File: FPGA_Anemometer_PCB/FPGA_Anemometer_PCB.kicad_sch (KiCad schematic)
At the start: 7 parts, among them J3 YO0221500000G, J4 YO0221500000G

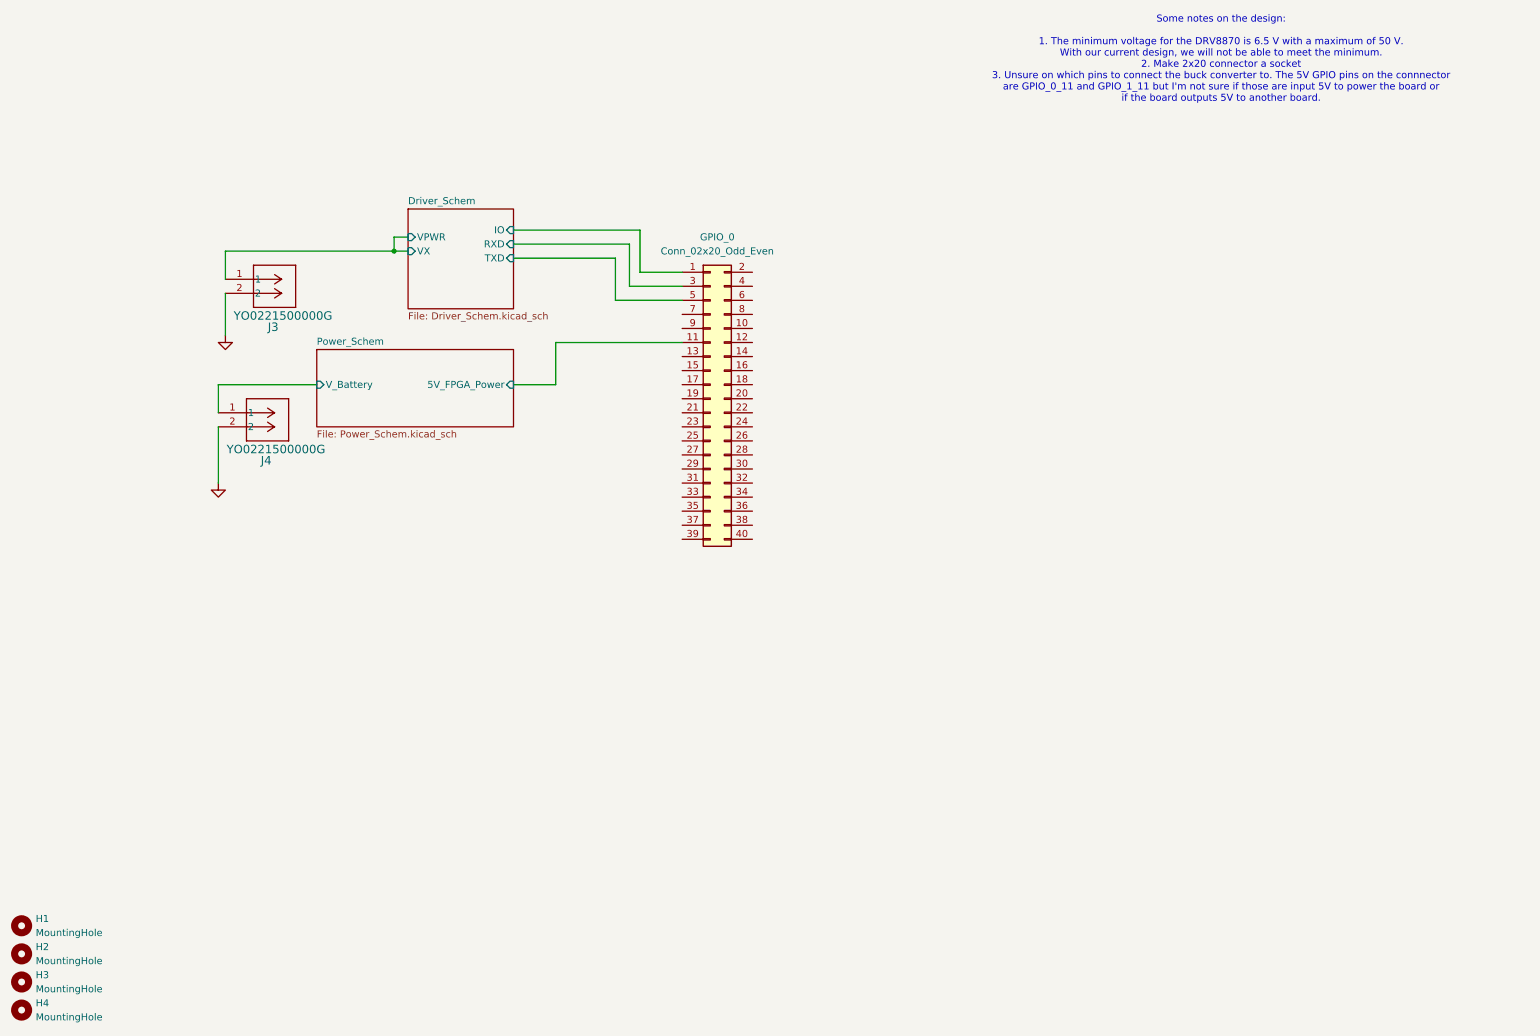
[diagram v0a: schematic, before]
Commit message: updated pcb
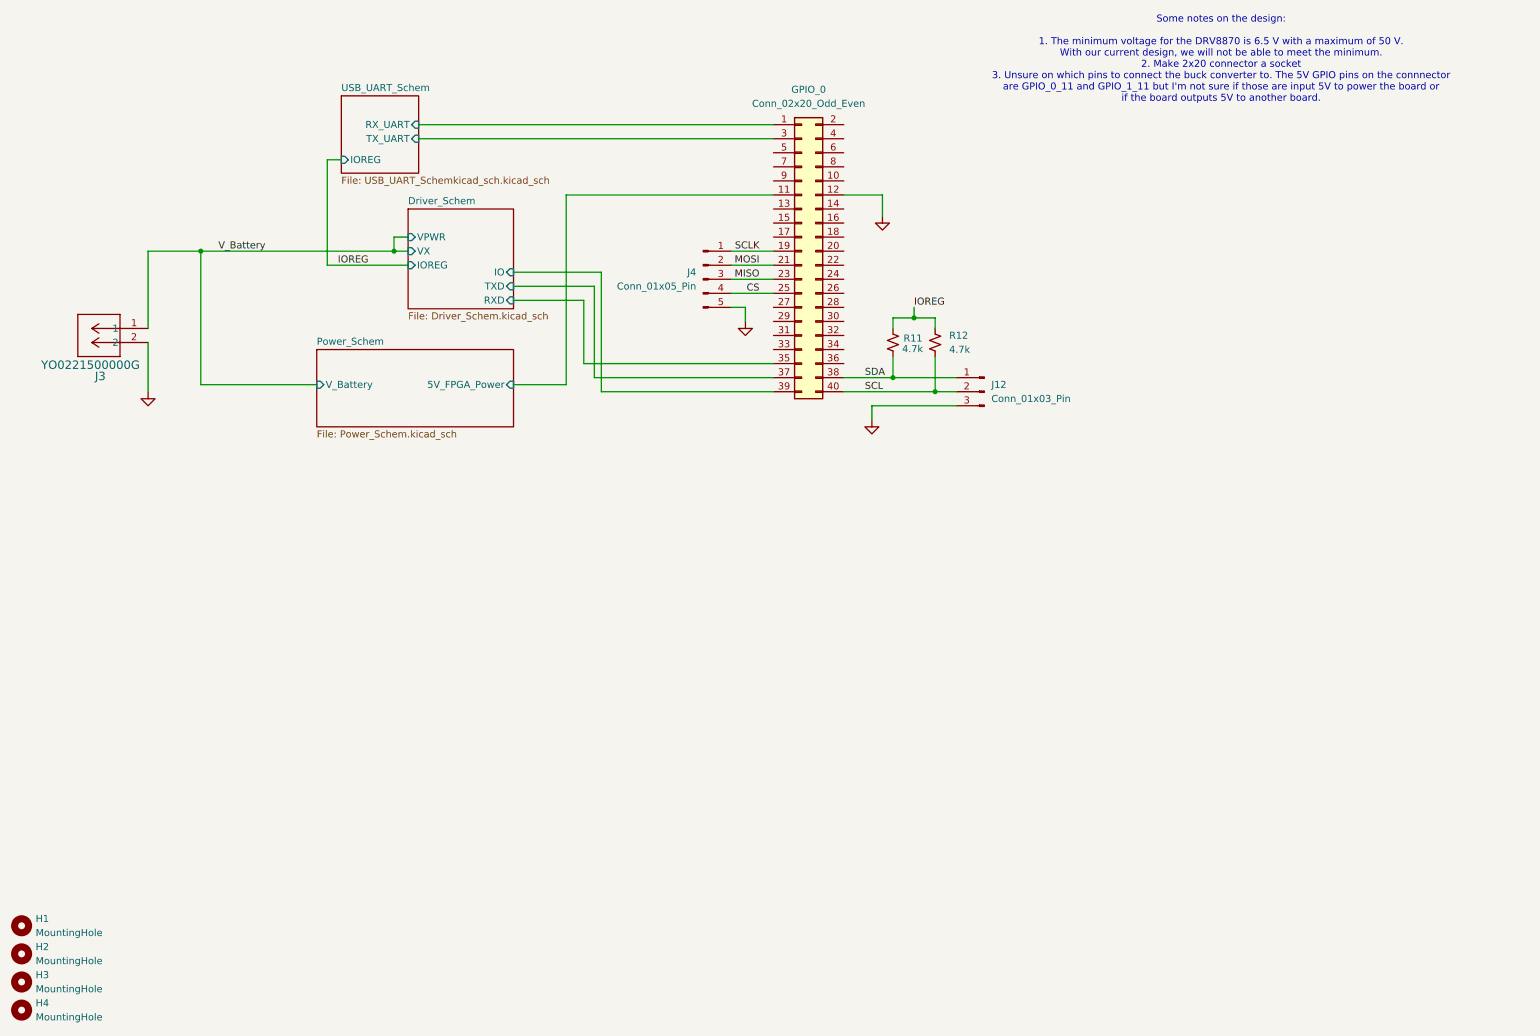
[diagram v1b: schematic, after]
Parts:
- removed J4: YO0221500000G, footprints:CONN_YO0221500000G_AMP, symbol 2026-01-23_14-54-26:YO0221500000G
- added J12: Conn_01x03_Pin, Connector_PinHeader_2.54mm:PinHeader_1x03_P2.54mm_Vertical, symbol Connector:Conn_01x03_Pin
- added J4: Conn_01x05_Pin, Connector_PinHeader_2.54mm:PinHeader_1x05_P2.54mm_Vertical, symbol Connector:Conn_01x05_Pin
- added R11, R12: 4.7k, Resistor_SMD:R_0805_2012Metric, symbol Device:R_Small_US
- J3: footprint footprints:CONN_YO0221500000G_AMP -> YO0221500000G:CONN_YO0221500000G_AMP
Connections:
- net Driver_Schem/IO: now also GPIO_0.39 (Pin_39); no longer GPIO_0.1 (Pin_1)
- net Driver_Schem/RXD: now also GPIO_0.35 (Pin_35); no longer GPIO_0.3 (Pin_3)
- net Driver_Schem/TXD: now also GPIO_0.37 (Pin_37); no longer GPIO_0.5 (Pin_5)
- net GND: now also GPIO_0.12 (Pin_12), J12.3 (Pin_3), J4.5 (Pin_5)
- net SCLK: now reaches GPIO_0.19 (Pin_19)
- net SCLK: now also J4.1 (Pin_1)
- net MOSI: now reaches GPIO_0.21 (Pin_21)
- net MOSI: now also J4.2 (Pin_2)
- net MISO: now reaches GPIO_0.23 (Pin_23)
- net MISO: now also J4.3 (Pin_3)
- net CS: now reaches GPIO_0.25 (Pin_25)
- net CS: now also J4.4 (Pin_4)
- net SDA: now reaches GPIO_0.38 (Pin_38)
- net SDA: now also J12.1 (Pin_1), R11.2
- net SCL: now reaches GPIO_0.40 (Pin_40)
- net SCL: now also J12.2 (Pin_2), R12.2
- net Driver_Schem/VPWR renamed V_Battery
- new net IOREG: R11.1, R12.1
- new net USB_UART_Schem/RX_UART: GPIO_0.1 (Pin_1)
- new net USB_UART_Schem/TX_UART: GPIO_0.3 (Pin_3)
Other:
- added sheet USB_UART_Schem (USB_UART_Schemkicad_sch.kicad_sch)
- sheet Driver_Schem ports: added IOREG; removed none
- moved on the sheet: GPIO_0, J3
